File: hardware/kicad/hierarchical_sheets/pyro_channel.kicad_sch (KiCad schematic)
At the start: 19 parts, among them J2 282834-4, U2 ZXCT1110W5-7, U3 SI9926CDY

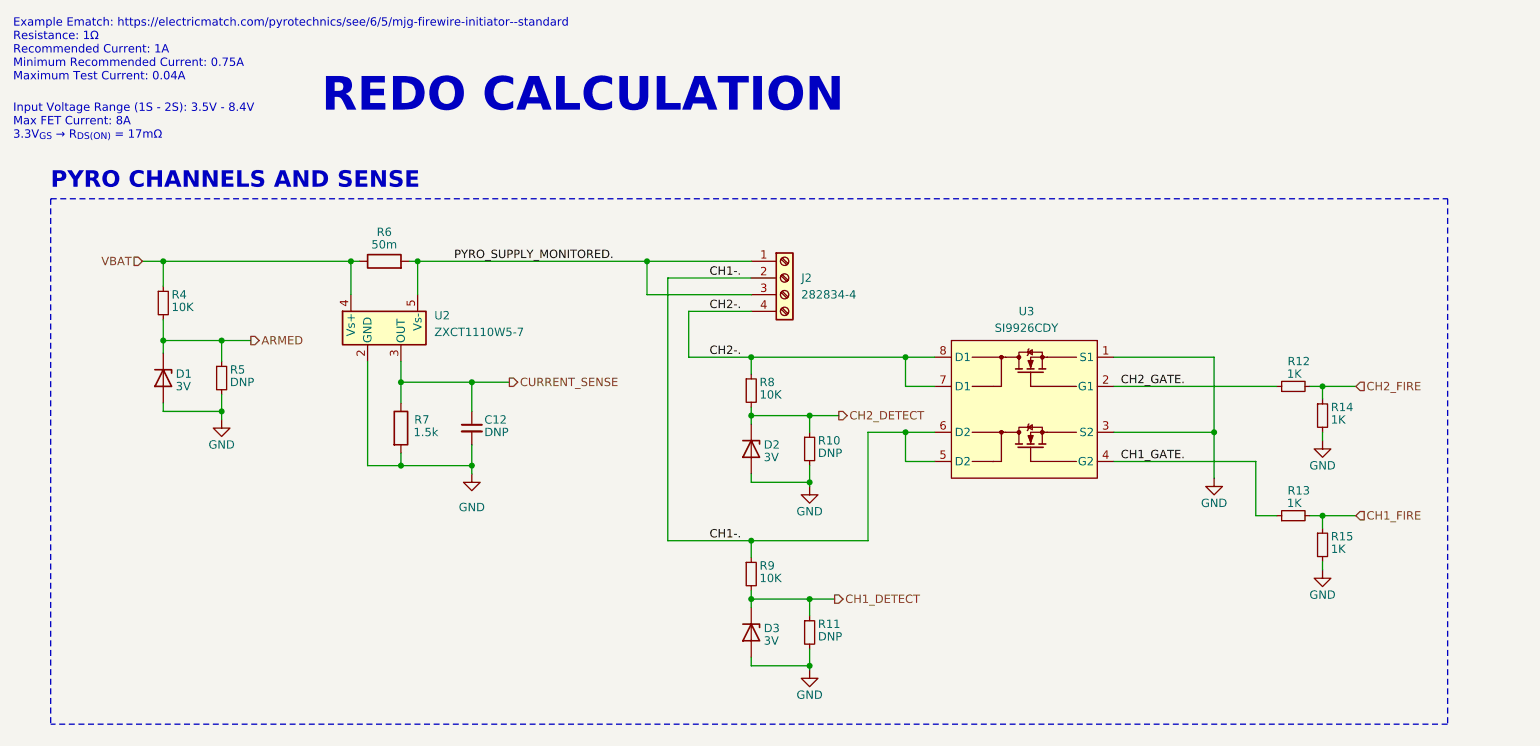
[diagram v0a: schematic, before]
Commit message: added power and checked schematics
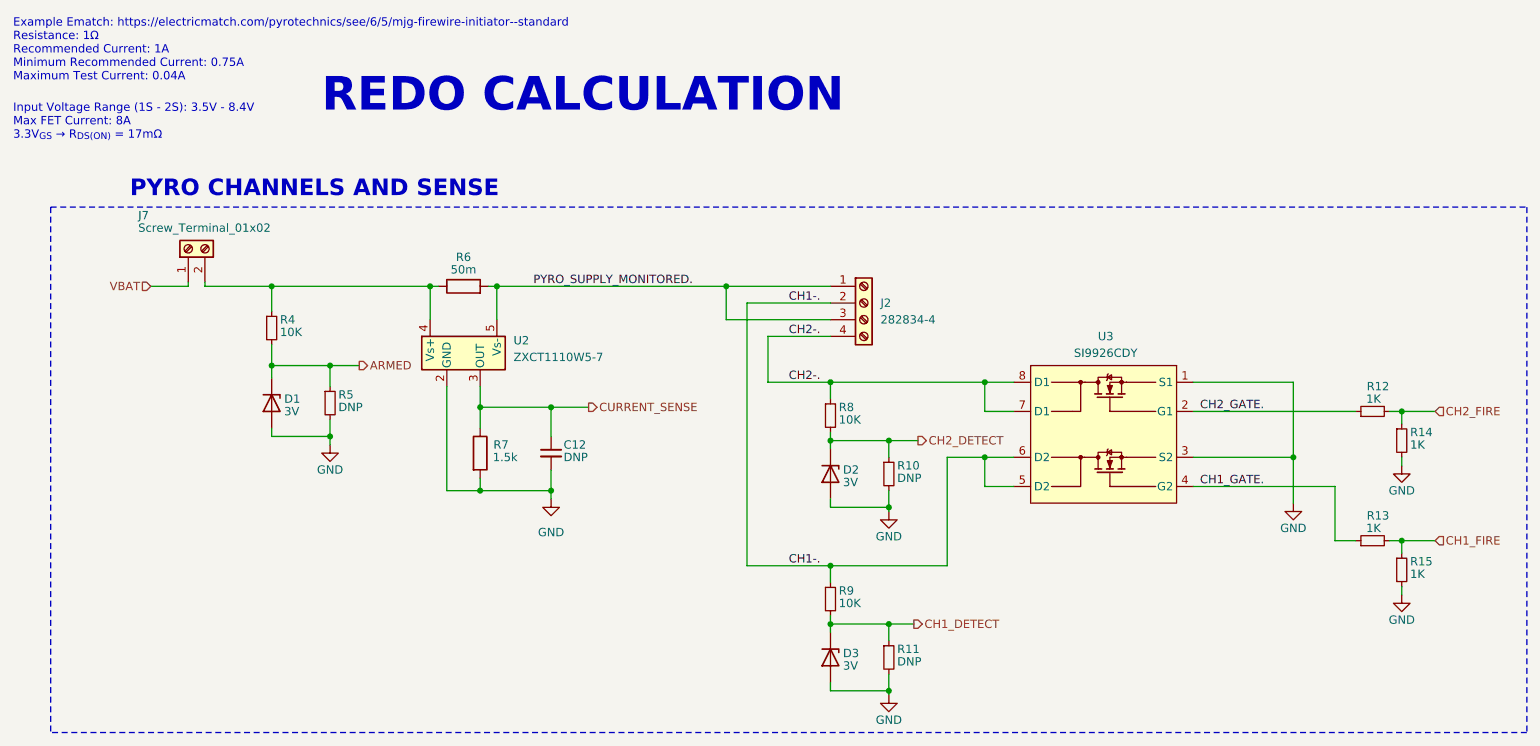
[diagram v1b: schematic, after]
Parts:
- added J7: Screw_Terminal_01x02, symbol Connector:Screw_Terminal_01x02
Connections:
- net VBAT: now also J7.1 (Pin_1); no longer R4.1, R6.1, U2.4 (Vs+)
- new net: J7.2 (Pin_2), R4.1, R6.1, U2.4 (Vs+)
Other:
- moved on the sheet: C12, D1, D2, D3, J2, R10, R11, R12, R13, R14, R15, R4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
